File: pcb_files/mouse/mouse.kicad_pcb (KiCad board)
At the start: 2 copper layers, 94.7 x 93.9 mm, 26 parts, among them M1 Motor_DC, M2 Motor_DC, M3 Motor_DC, Q0 Q_Photo_NPN, Q1 Q_Photo_NPN, Q2 Q_Photo_NPN, Q3 Q_Photo_NPN, U1 Teensy3.2, U2 SN754410NE, U3 LM1084-5.0, U4 Encoder_3081, U5 Encoder_3081, U6 NRF24L01_Breakout

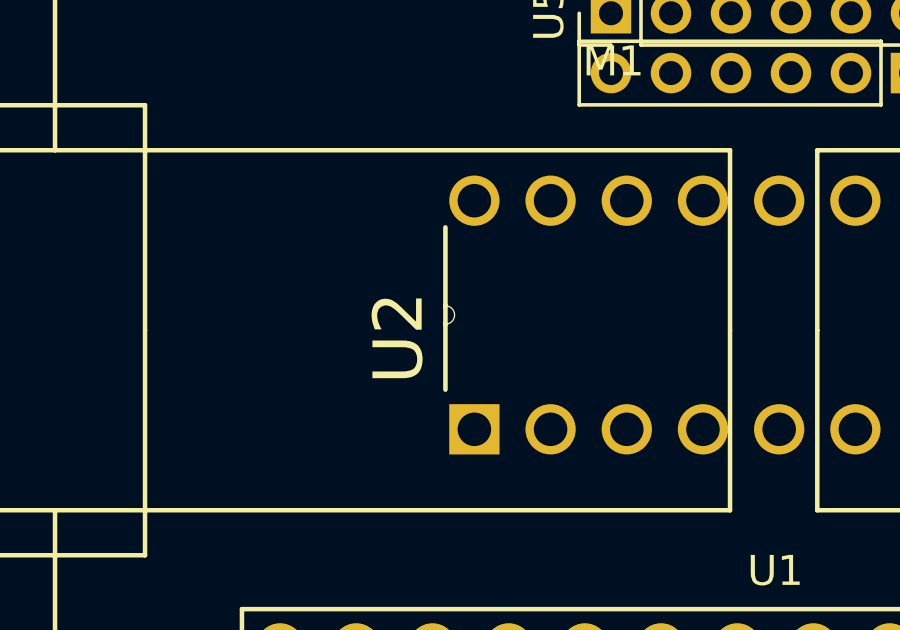
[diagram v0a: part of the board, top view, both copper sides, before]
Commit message: removed wirless module
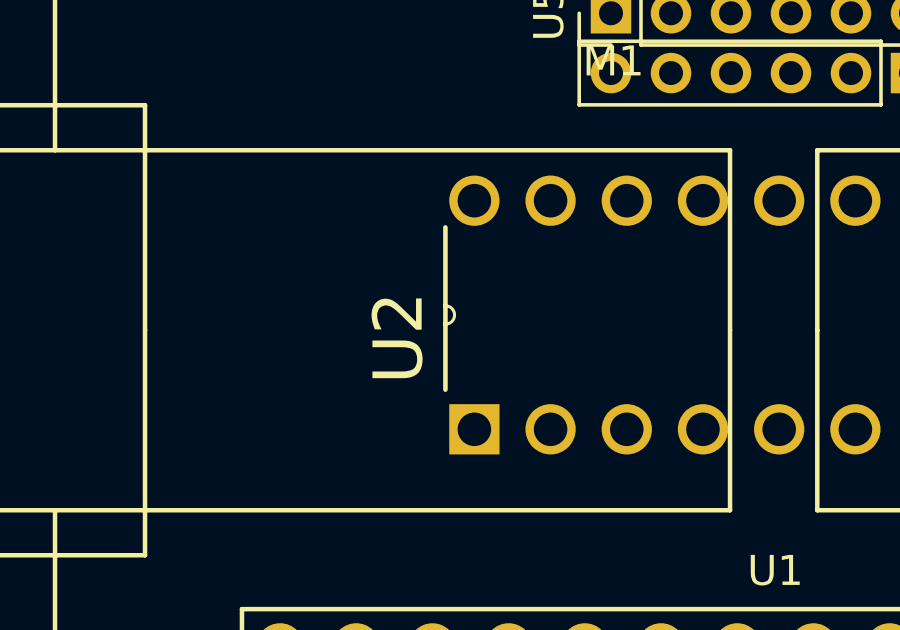
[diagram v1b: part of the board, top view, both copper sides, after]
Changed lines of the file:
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@@
-(kicad_pcb (version 20171130) (host pcbnew "(5.0.0-3-g5ebb6b6)")
+(kicad_pcb (version 20171130) (host pcbnew "(5.1.2)-2")
   (general
     (thickness 1.6)
@@
     (zone_45_only no)
     (trace_min 0.2)
-    (segment_width 0.2)
-    (edge_width 0.15)
     (via_size 0.8)
     (via_drill 0.4)
@@
     (uvia_min_size 0.2)
     (uvia_min_drill 0.1)
+    (edge_width 0.15)
+    (segment_width 0.2)
     (pcb_text_width 0.3)
     (pcb_text_size 1.5 1.5)
@@
     (pad_to_mask_clearance 0.2)
     (aux_axis_origin 0 0)
-    (visible_elements FFFFFF7F)
+    (visible_elements 7FFFFFFF)
     (pcbplotparams
       (layerselection 0x010fc_ffffffff)
@@
     (fp_line (start -3.5052 -18.7452) (end -4.1148 -18.7452) (layer F.SilkS) (width 0.1524))
     (fp_line (start -4.1148 -18.7452) (end -6.2992 -18.7452) (layer F.SilkS) (width 0.1524))
-    (fp_arc (start -3.81 -18.7452) (end -4.1148 -18.7452) (angle -180) (layer F.SilkS) (width 0))
+    (fp_arc (start -3.81 -18.7452) (end -4.1148 -18.7452) (angle -180) (layer F.SilkS) (width 0.1))
     (fp_line (start -7.112 -17.2212) (end -7.112 -18.3388) (layer Eco2.User) (width 0.1524))
     (fp_line (start -7.112 -18.3388) (end -8.1788 -18.3388) (layer Eco2.User) (width 0.1524))
@@
     (fp_line (start -4.1148 -18.7452) (end -7.112 -18.7452) (layer Eco2.User) (width 0.1524))
     (fp_line (start -7.112 -18.7452) (end -7.112 0.9652) (layer Eco2.User) (width 0.1524))
-    (fp_arc (start -3.81 -18.7452) (end -4.1148 -18.7452) (angle -180) (layer Eco2.User) (width 0))
+    (fp_arc (start -3.81 -18.7452) (end -4.1148 -18.7452) (angle -180) (layer Eco2.User) (width 0.1))
     (pad 1 thru_hole rect (at -7.62 -17.78 90) (size 1.6764 1.6764) (drill 1.1176) (layers *.Cu *.Mask)
       (net 24 /M1_speed))
